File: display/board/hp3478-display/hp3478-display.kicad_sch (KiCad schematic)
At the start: 24 parts, among them J1 SFV10R-1ST, J2 DNP, U1 PIC16F15274-I/MP, U2 DNP

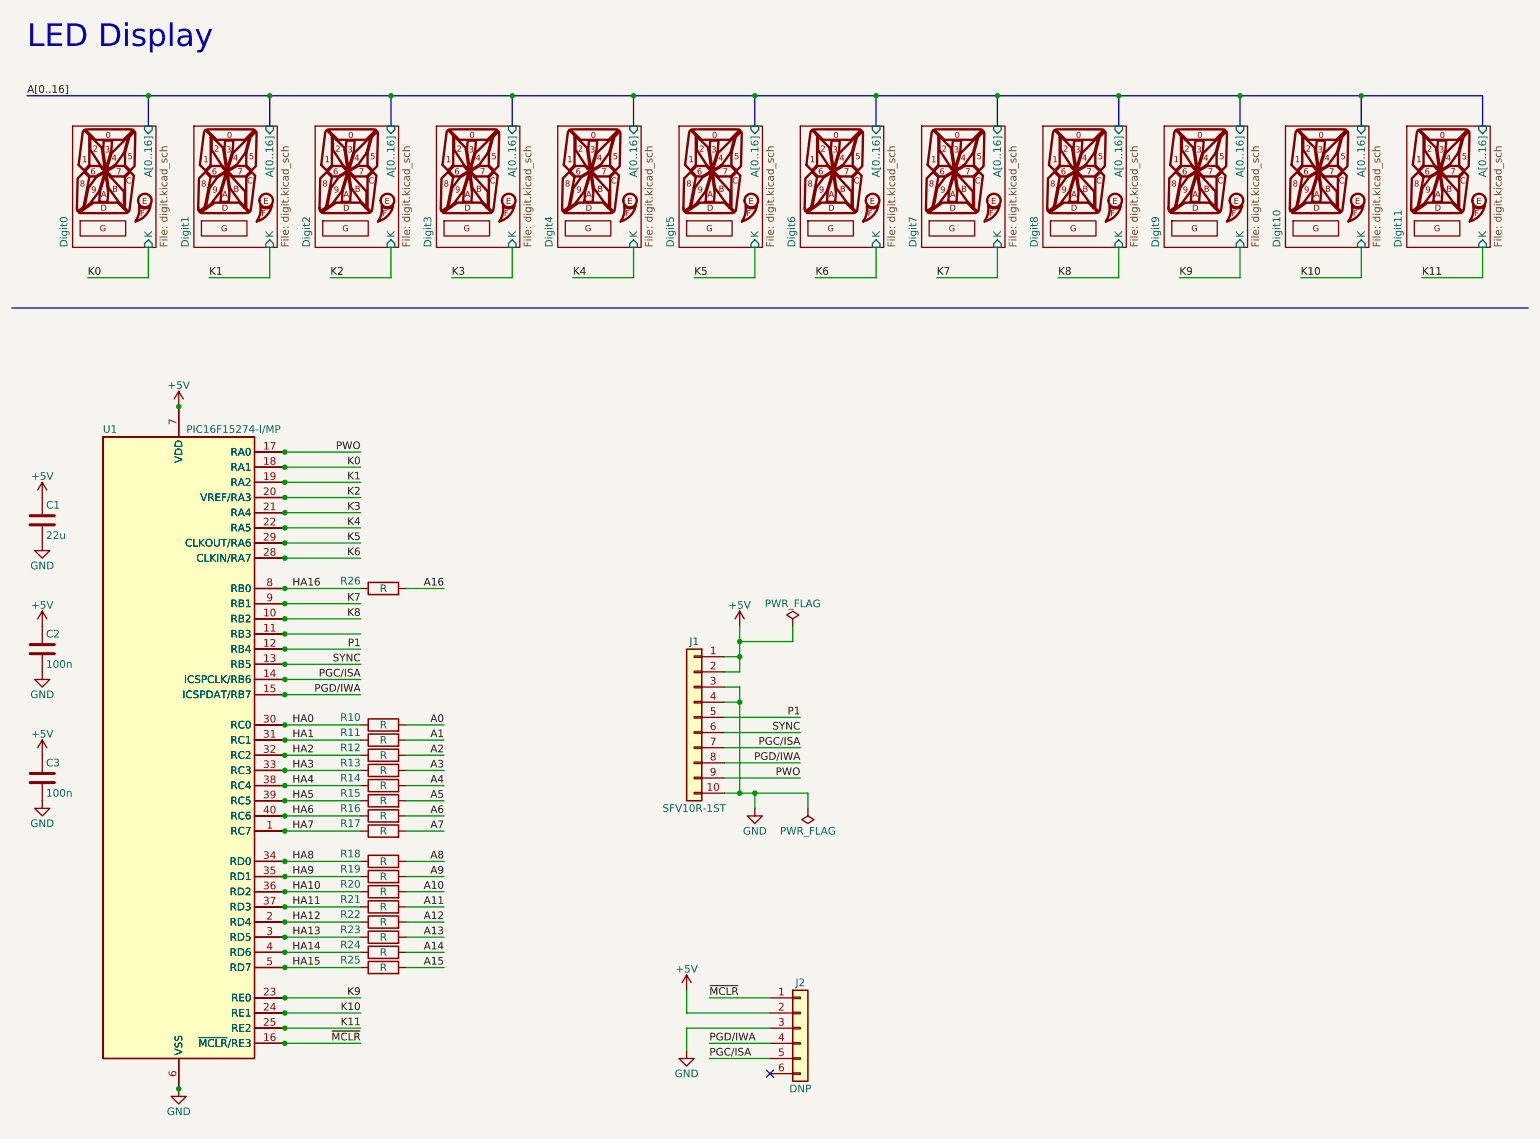
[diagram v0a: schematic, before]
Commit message: Reorganize schematic.
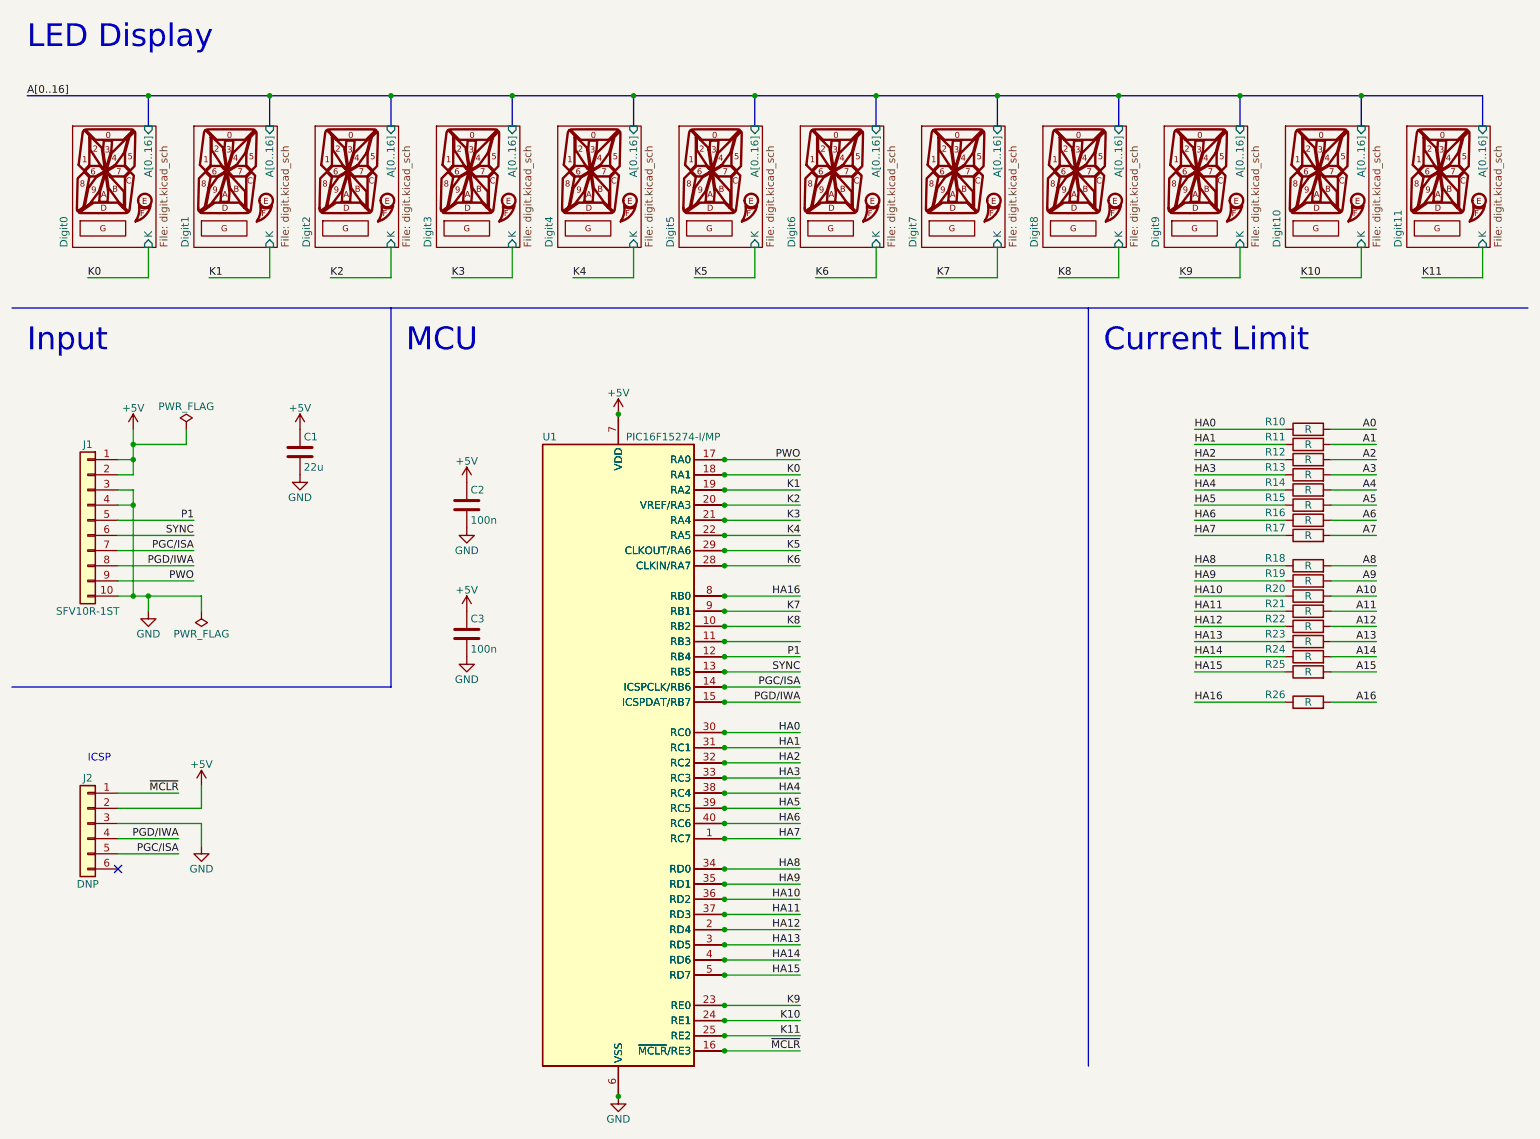
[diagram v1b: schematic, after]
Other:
- note added: "Current Limit"
- note added: "ICSP"
- note added: "Input"
- note added: "MCU"
- moved on the sheet: C1, C2, C3, J1, J2, R10, R11, R12, R13, R14, R15, R16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
